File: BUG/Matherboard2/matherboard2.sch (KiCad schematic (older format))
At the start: 38 parts, among them CON1 BARREL_JACK, J1 RJ12, J2 RJ12, J3 RJ12, P1 ON/OFF, P2 FW, P3 RXTX, U1 BUTTON, U2 AP1117-5, U3 ESP-201, U4 AP1117-3

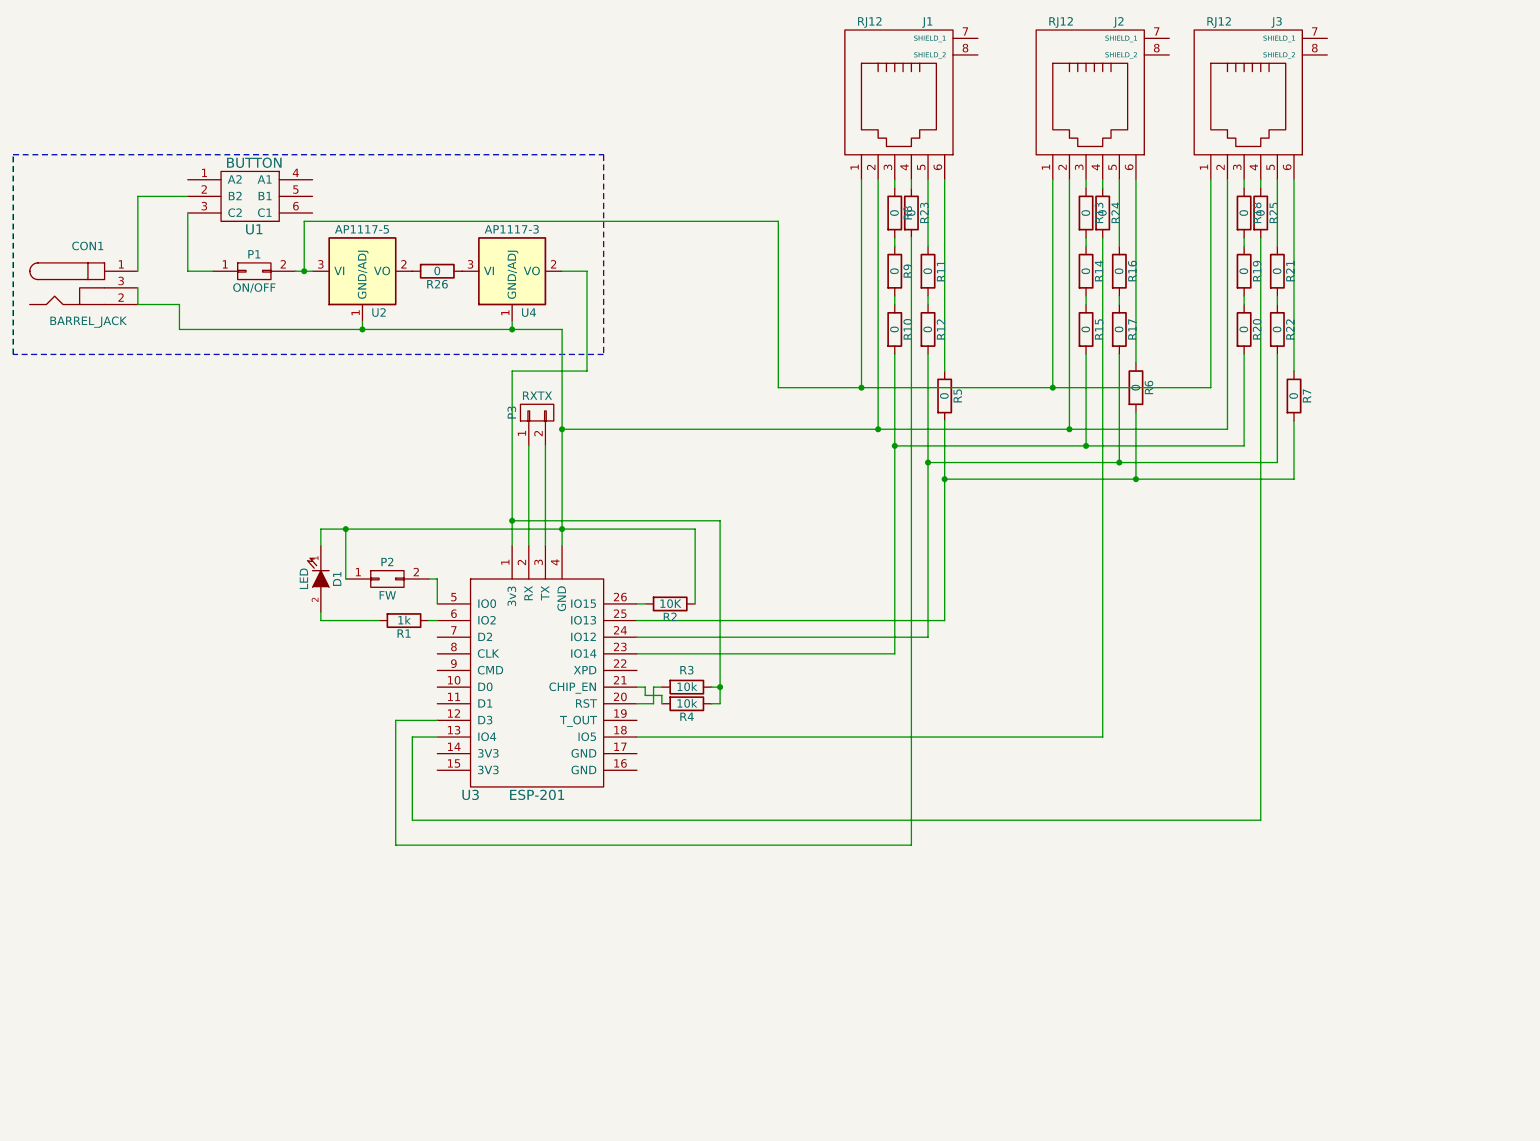
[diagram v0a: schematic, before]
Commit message: Many uodates
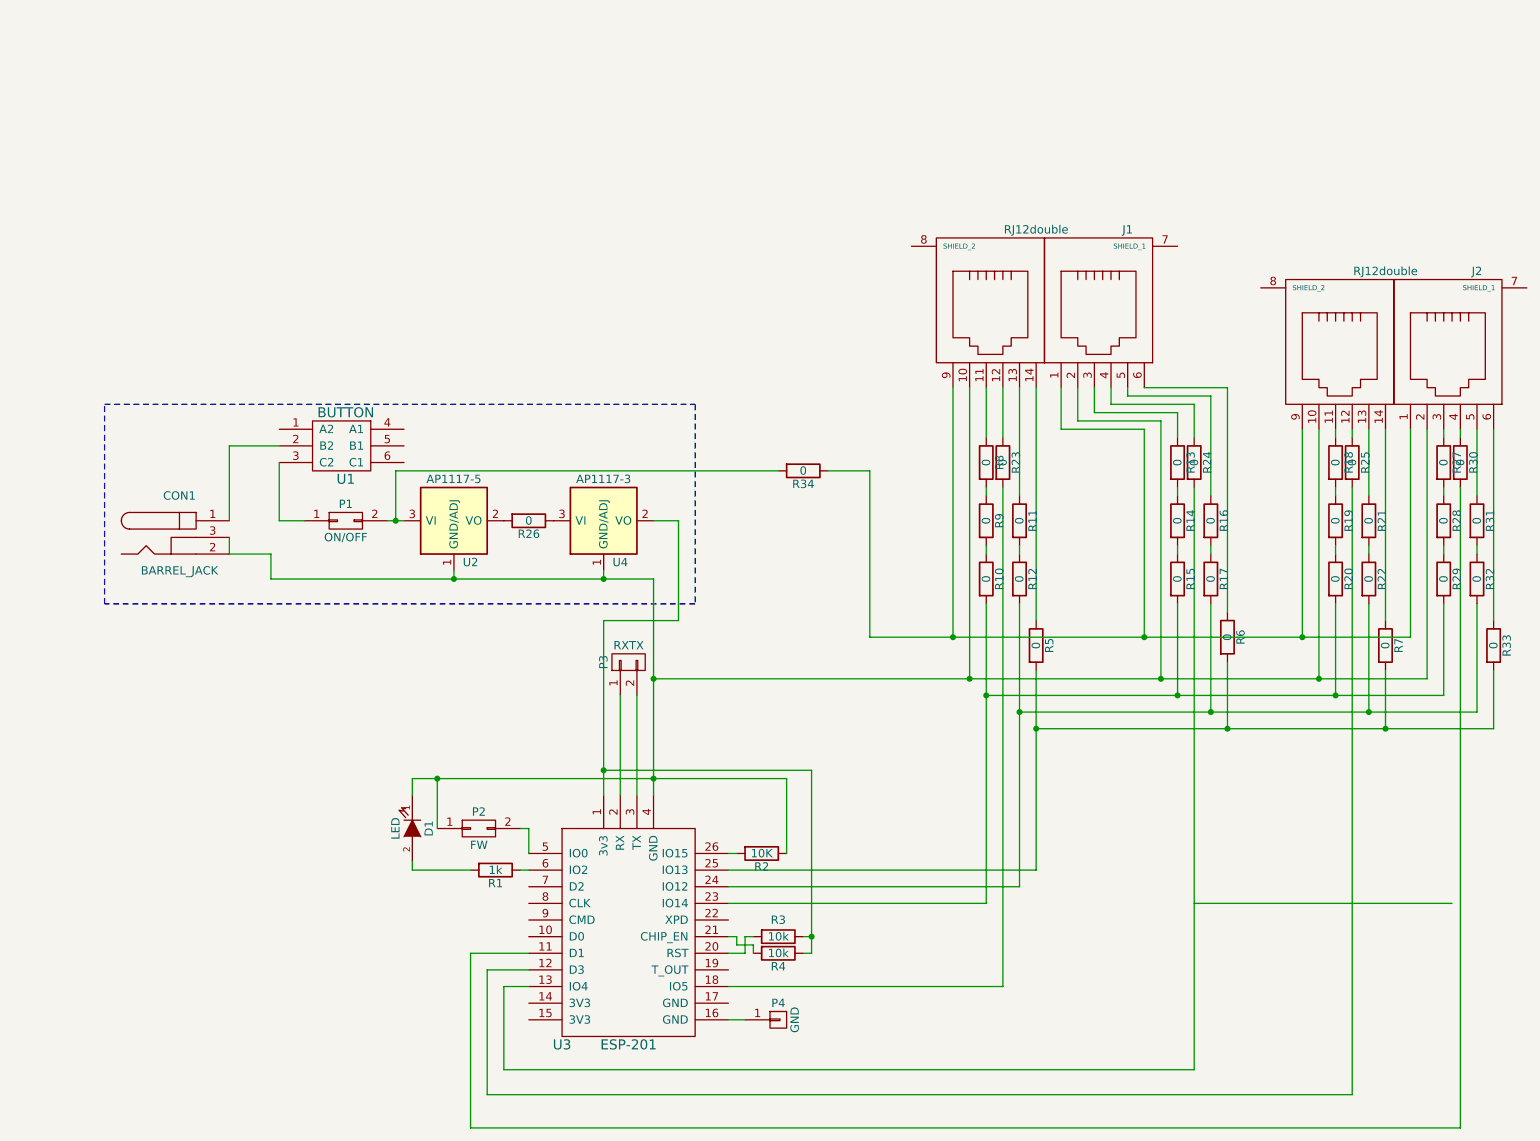
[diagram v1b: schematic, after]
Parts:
- removed J1, J2, J3: RJ12, Connect:RJ12_E, symbol RJ12
- added J1, J2: RJ12double, bugs:RJ12double, symbol RJ12double
- added P4: GND, Pin_Headers:Pin_Header_Straight_1x01, symbol CONN_01X01
- added R27, R28, R29, R30, R31, R32, R33, R34: 0, Resistors_SMD:R_1206, symbol R
- U2, U4: footprint Buttons_Switches_ThroughHole:SW_Micro_SPST -> bugs:SMD-stab
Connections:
- net at CON1.2, CON1.3, D1.1 (K)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: now also J1.10, J1.2, J2.10, J2.2
- net at U3.11 (D1): now also R30.2
- net at U3.12 (D3): now also R25.2; no longer R23.2
- net at U3.13 (IO4): now also R24.2; no longer R25.2
- net at U3.16 (GND): now also P4.1 (P1)
- net at U3.18 (IO5): now also R23.2; no longer R24.2
- net at R10.2, R15.2, R20.2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: now also R29.2
- net at R12.2, R17.2, R22.2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: now also R32.2
- net at R5.2, R6.2, R7.2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: now also R33.2
- net at P1.2 (P2), U2.3 (VI): now also R34.2
- net at R7.1: now also J2.14
- net at R6.1: now also J1.6
- net at R5.1: now also J1.14
- net at R8.1: now also J1.11
- net at R23.1: now also J1.12
- net at R11.1: now also J1.13
- net at R13.1: now also J1.3
- net at R24.1: now also J1.4
- net at R16.1: now also J1.5
- net at R18.1: now also J2.11
- net at R25.1: now also J2.12
- net at R21.1: now also J2.13
- new net: J1.1, J1.9, J2.1, J2.9, R34.1
- new net: J2.3, R27.1
- new net: J2.4, R30.1
- new net: J2.5, R31.1
- new net: J2.6, R33.1
- new net: R31.2, R32.1
- new net: R27.2, R28.1
- new net: R28.2, R29.1
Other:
- moved on the sheet: CON1, D1, P1, P2, P3, R1, R10, R11, R12, R13, R14, R15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
